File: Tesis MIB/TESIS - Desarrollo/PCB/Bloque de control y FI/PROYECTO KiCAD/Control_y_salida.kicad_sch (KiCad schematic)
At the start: 30 parts, among them J5 FSR_b, J6 FSR_a, Q1 BF422, Q2 BF421, Q3 BF557, Q4 BC547, Q5 BF421, Q6 BF422, SW1 Decr, SW2 Inc, SW3 Acept, U1 LCD-016N002L, U2 PSoC4_kit049_(CY8C4245AXI-483), U3 TL082

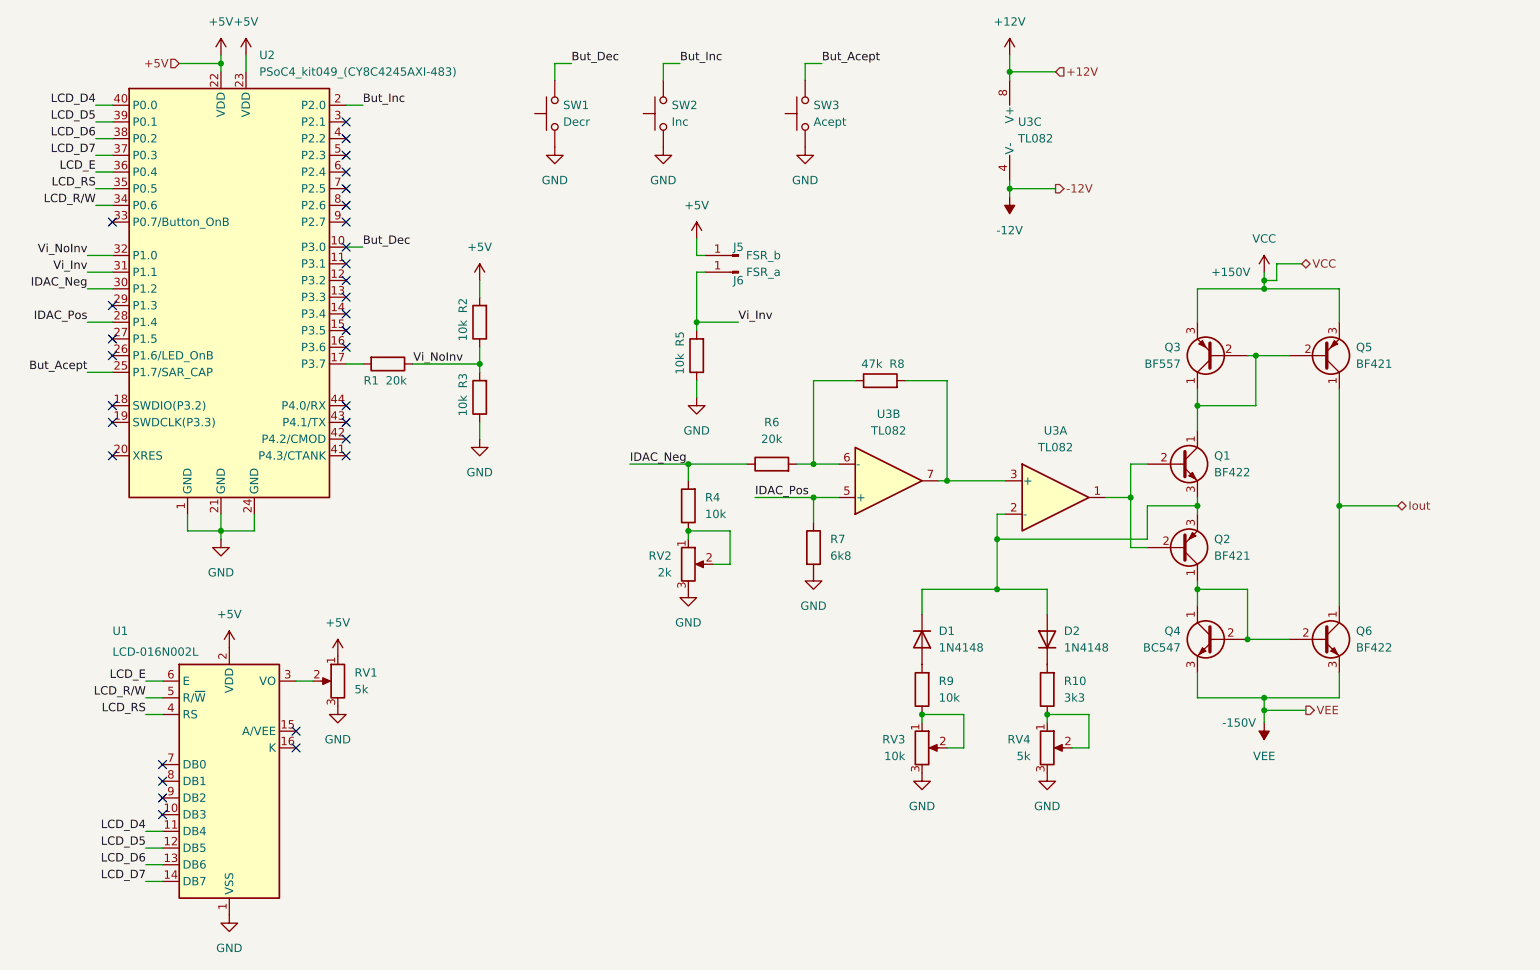
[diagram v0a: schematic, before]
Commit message: Actualiza avances
Se incorporan varios artículos de referencia y se actualiza el documento de Tesis con el Cap 1 (pag. 19 a 39).
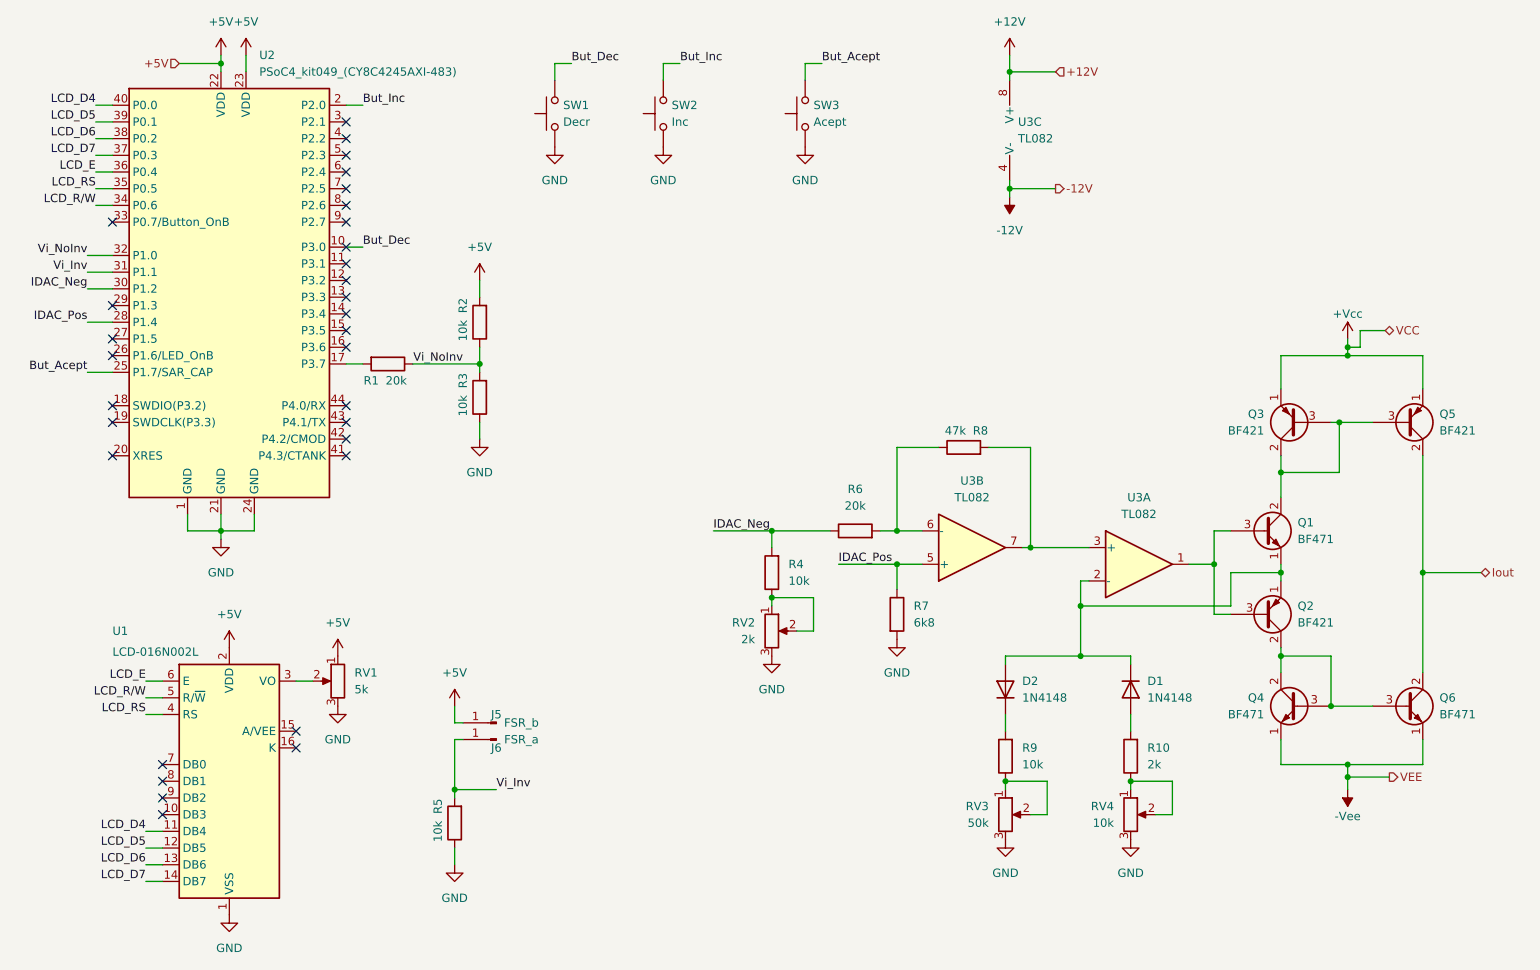
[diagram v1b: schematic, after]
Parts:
- Q1, Q6: value BF422 -> BF471
- Q3: value BF557 -> BF421
- Q4: value BC547 -> BF471
- R10: value 3k3 -> 2k
- RV3: value 10k -> 50k
- RV4: value 5k -> 10k
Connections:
- net Iout: now also Q5.2 (C), Q6.2 (C); no longer Q5.1 (C), Q6.1 (C)
- net VCC: now also Q3.1 (E), Q5.1 (E); no longer Q3.3 (E), Q5.3 (E)
- net VEE: now also Q4.1 (E), Q6.1 (E); no longer Q4.3 (E), Q6.3 (E)
- net at D2.1 (K): now also R9.2; no longer R10.2
- net at D1.1 (K), D2.2 (A), U3.2 (-): now also Q1.1 (E), Q2.1 (E); no longer Q1.3 (E), Q2.3 (E)
- net at D1.2 (A): now also R10.2; no longer R9.2
- new net: Q1.2 (C), Q3.2 (C), Q3.3 (B), Q5.3 (B)
- new net: Q1.3 (B), Q2.3 (B), U3.1
- new net: Q2.2 (C), Q4.2 (C), Q4.3 (B), Q6.3 (B)
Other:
- moved on the sheet: D1, D2, J5, J6, Q1, Q5, R10, R4, R5, R6, R7, R8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
